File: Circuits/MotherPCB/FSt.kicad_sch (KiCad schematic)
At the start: 0 parts

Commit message: Done for the night
Finished up thermocouple differential communication and every other module apart from PTs and Oil Injector.

Good night.
oh wait
It's 4:00 am.
Good morning
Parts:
- added J5: PINHD_1x4_Male, Connector_PinHeader_2.54mm:PinHeader_1x04_P2.54mm_Vertical, symbol PCM_SL_Pin_Headers:PINHD_1x4_Male
- added J6: XT60-M, XT60-M:AMASS_XT60-M, symbol XT60-M:XT60-M
- added J7: PINHD_2x3_Female, Connector_PinSocket_2.54mm:PinSocket_2x03_P2.54mm_Vertical, symbol PCM_SL_Pin_Headers:PINHD_2x3_Female
- added U1: A4988, PCM_SL_Breakout_Boards:A4988_Breakout, symbol PCM_SL_Breakout_Boards:A4988
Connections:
- new net: J7.2, U1.4 (MS3)
- new net: J7.4, U1.3 (MS2)
- new net: J7.6, U1.2 (MS1)
- new net: J5.1, U1.14 (B2)
- new net: J5.2, U1.13 (A2)
- new net: J5.3, U1.12 (A1)
- new net: J5.4, U1.11 (B1)
- new net: J6.P (POS), U1.16 (VMOT)
- new net 3V3: J7.1, J7.3, J7.5, U1.10 (VDD)
- new net DIR: U1.8 (DIR)
- new net EN: U1.1 (EN)
- new net GND: J6.N (NEG), U1.15 (GND), U1.9 (GND)
- new net STP: U1.7 (STEP)

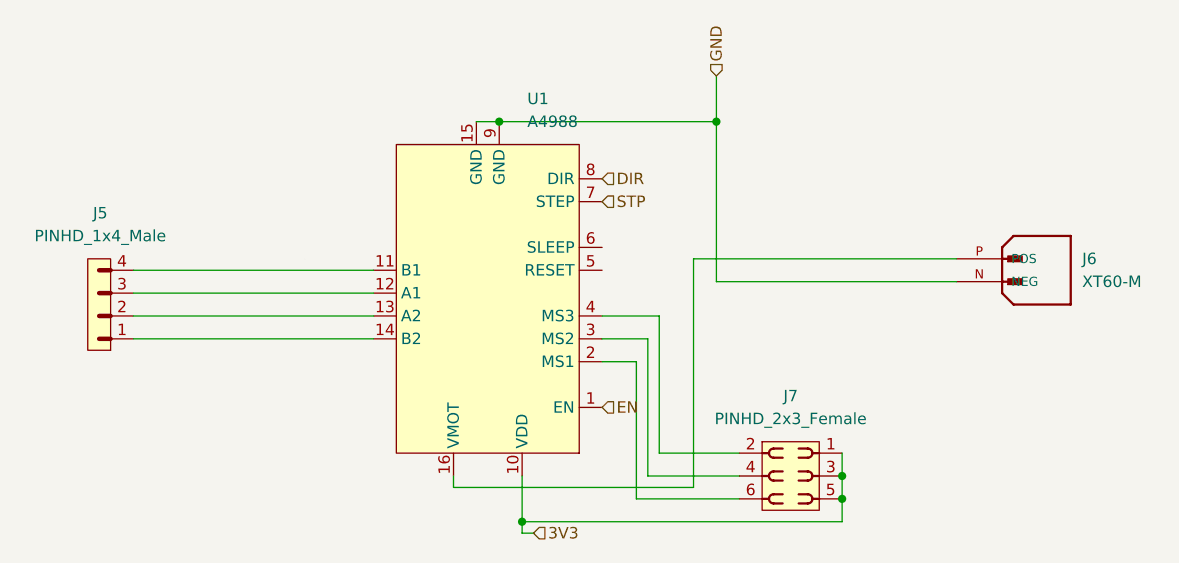
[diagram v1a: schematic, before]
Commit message: pcb completed with a clean DRC
first one it is let us pray it works
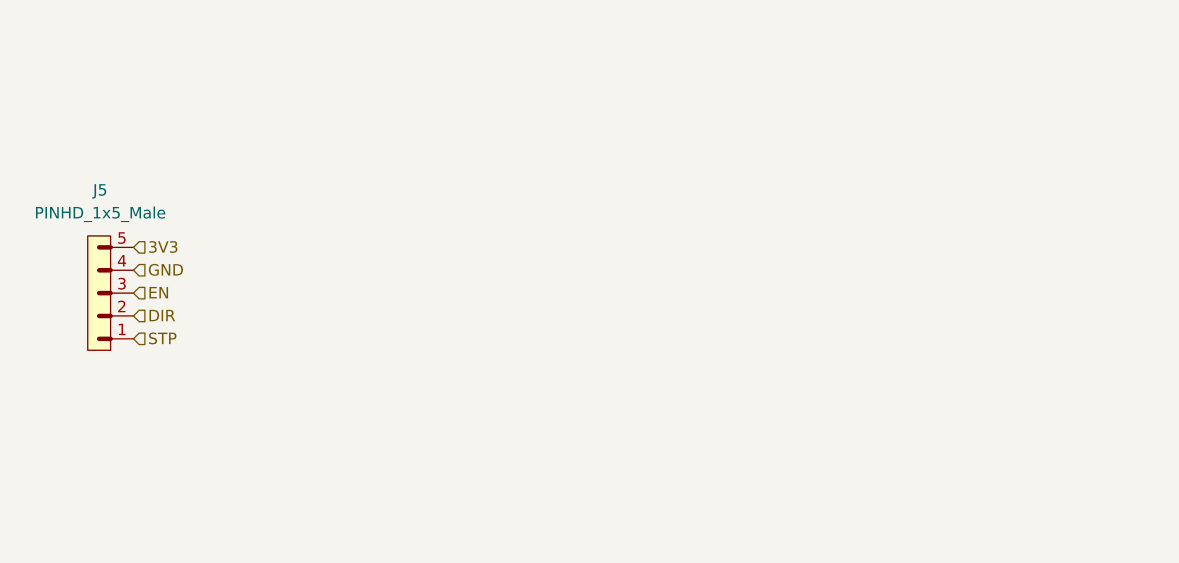
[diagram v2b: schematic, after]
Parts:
- removed J5: PINHD_1x4_Male, Connector_PinHeader_2.54mm:PinHeader_1x04_P2.54mm_Vertical, symbol PCM_SL_Pin_Headers:PINHD_1x4_Male
- removed J6: XT60-M, XT60-M:AMASS_XT60-M, symbol XT60-M:XT60-M
- removed J7: PINHD_2x3_Female, Connector_PinSocket_2.54mm:PinSocket_2x03_P2.54mm_Vertical, symbol PCM_SL_Pin_Headers:PINHD_2x3_Female
- removed U1: A4988, PCM_SL_Breakout_Boards:A4988_Breakout, symbol PCM_SL_Breakout_Boards:A4988
- added J5: PINHD_1x5_Male, Connector_PinHeader_2.54mm:PinHeader_1x05_P2.54mm_Vertical, symbol PCM_SL_Pin_Headers:PINHD_1x5_Male
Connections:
- net 3V3: now also J5.5
- net DIR: now also J5.2
- net EN: now also J5.3
- net GND: now also J5.4
- net STP: now also J5.1
